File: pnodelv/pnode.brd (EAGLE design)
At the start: 50 x 23 mm, 42 parts, among them IC2 HTU21D, IC3 SI4012, J1 SWD_SHROUD_SMD

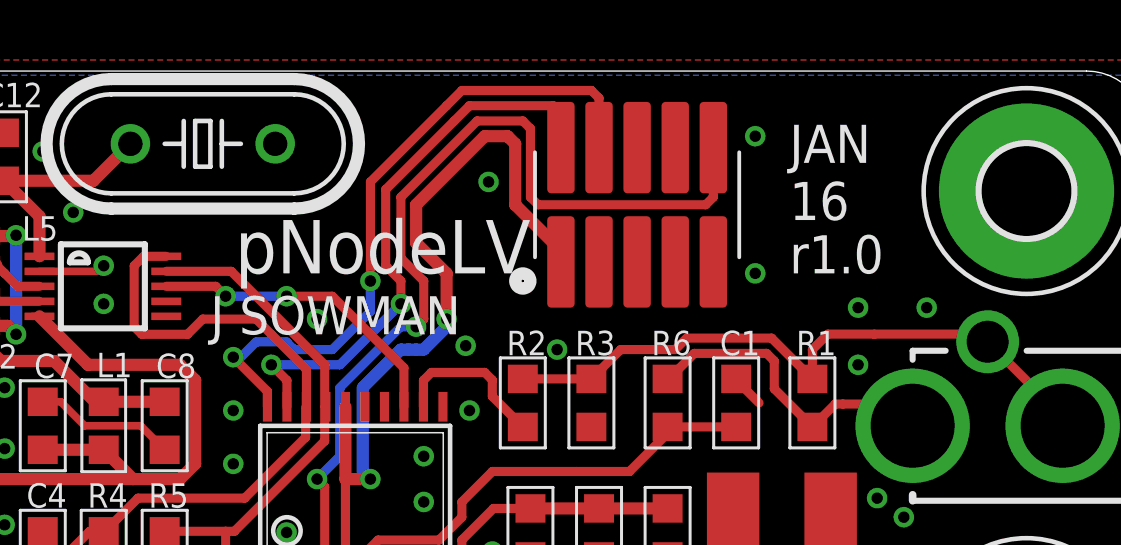
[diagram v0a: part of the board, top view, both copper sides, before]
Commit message: tidying silk again
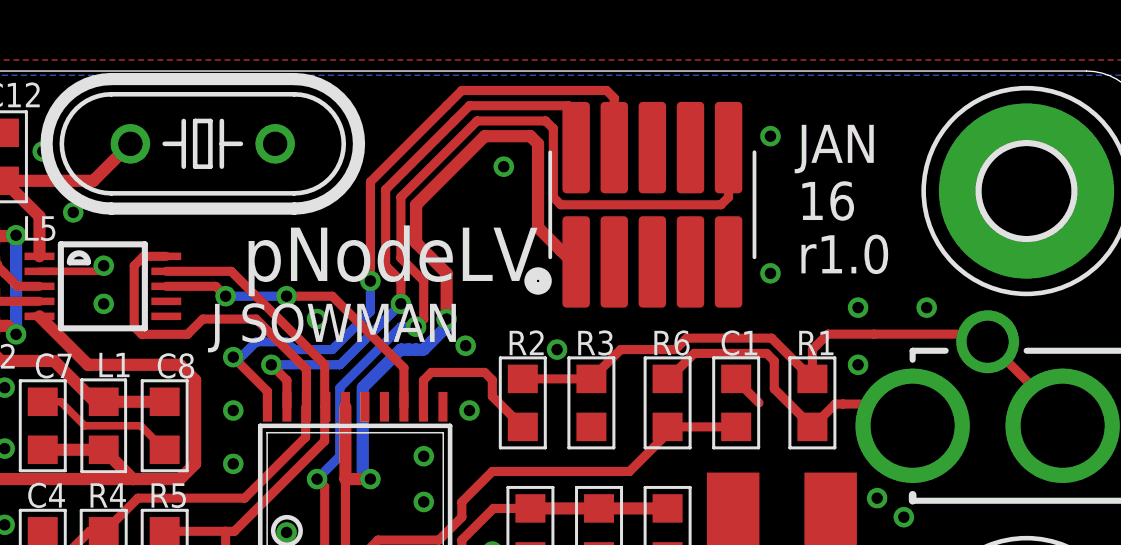
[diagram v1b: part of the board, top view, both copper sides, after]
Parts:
- moved J1 0.51 mm to (33.5, 18.5)
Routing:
- net +3V3: track 92.0 -> 92.6 mm
- net SWCLK: track 22.5 -> 23.0 mm
- net SWDAT: track 19.0 -> 19.6 mm
- net NRST: track 30.8 -> 31.3 mm
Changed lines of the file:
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@@
 <wire x1="50" y1="21" x2="48" y2="23" width="0" layer="20" curve="90"/>
 <text x="11.176" y="2.032" size="1.27" layer="21" font="vector" ratio="15" rot="R90">M0JSN</text>
-<text x="18.796" y="14.224" size="1.27" layer="21" font="vector" ratio="15">J SOWMAN</text>
-<text x="38.1" y="18.034" size="1.27" layer="21" font="vector" ratio="15">JAN
+<text x="18.796" y="13.97" size="1.27" layer="21" font="vector" ratio="15">J SOWMAN</text>
+<text x="38.354" y="18.034" size="1.27" layer="21" font="vector" ratio="15">JAN
 16</text>
 <text x="9.398" y="0.508" size="1.27" layer="21" font="vector" ratio="15" rot="R90">UKHASnet</text>
 <text x="36.83" y="0.254" size="1.27" layer="21" font="vector" ratio="15">1.5V</text>
-<text x="29.464" y="18.034" size="1.778" layer="21" font="vector" ratio="15" rot="R180">pNodeLV</text>
+<text x="29.718" y="17.78" size="1.778" layer="21" font="vector" ratio="15" rot="R180">pNodeLV</text>
 <text x="33.02" y="5.842" size="2.54" layer="22" font="vector" ratio="15" rot="MR0">pNodeLV</text>
 <text x="34.544" y="1.778" size="2.54" layer="22" font="vector" ratio="15" rot="MR0">J SOWMAN</text>
 <text x="9.652" y="18.542" size="1.27" layer="22" font="vector" ratio="15" rot="MR270">jonsowman.com</text>
-<text x="38.1" y="16.256" size="1.27" layer="21" font="vector" ratio="15">r1.0</text>
+<text x="38.354" y="16.256" size="1.27" layer="21" font="vector" ratio="15">r1.0</text>
 </plain>
 <attributes>
@@
 </element>
 <element name="L6" library="jonsowman" package="BOURNS_SDE0403A" value="4.7u" x="37.846" y="7.366"/>
-<element name="J1" library="dtb" package="SWD_SMD_SHROUD" value="SWD_SHROUD_SMD" x="33.02" y="18.542"/>
+<element name="J1" library="dtb" package="SWD_SMD_SHROUD" value="SWD_SHROUD_SMD" x="33.528" y="18.542"/>
 </elements>
 <signals>
@@
 <wire x1="36.322" y1="12.738" x2="36.322" y2="12.7" width="0.3048" layer="1"/>
 <wire x1="36.322" y1="12.7" x2="37.084" y2="11.938" width="0.3048" layer="1"/>
-<via x="28.067" y="19.304" extent="1-16" drill="0.381"/>
+<via x="28.575" y="19.812" extent="1-16" drill="0.381"/>
 <via x="27.305" y="13.843" extent="1-16" drill="0.381"/>
-<via x="36.957" y="20.828" extent="1-16" drill="0.381"/>
-<via x="36.957" y="16.256" extent="1-16" drill="0.381"/>
+<via x="37.465" y="20.828" extent="1-16" drill="0.381"/>
+<via x="37.465" y="16.256" extent="1-16" drill="0.381"/>
 </signal>
 <signal name="+3V3">
@@
 <wire x1="25.108" y1="1.956" x2="25.146" y2="1.994" width="0.4064" layer="1"/>
 <contactref element="J1" pad="1"/>
-<wire x1="30.48" y1="16.637" x2="30.48" y2="16.764" width="0.4064" layer="1"/>
-<wire x1="30.48" y1="16.637" x2="30.48" y2="17.018" width="0.4064" layer="1"/>
-<wire x1="30.48" y1="17.018" x2="28.956" y2="18.542" width="0.4064" layer="1"/>
-<wire x1="28.956" y1="18.542" x2="28.956" y2="20.574" width="0.4064" layer="1"/>
-<wire x1="28.956" y1="20.574" x2="28.702" y2="20.828" width="0.4064" layer="1"/>
-<wire x1="28.702" y1="20.828" x2="27.94" y2="20.828" width="0.4064" layer="1"/>
+<wire x1="30.48" y1="17.018" x2="29.718" y2="17.78" width="0.4064" layer="1"/>
+<wire x1="29.718" y1="17.78" x2="29.718" y2="20.574" width="0.4064" layer="1"/>
+<wire x1="29.718" y1="20.574" x2="29.464" y2="20.828" width="0.4064" layer="1"/>
+<wire x1="29.464" y1="20.828" x2="27.94" y2="20.828" width="0.4064" layer="1"/>
 <wire x1="27.94" y1="20.828" x2="25.654" y2="18.542" width="0.4064" layer="1"/>
 <wire x1="25.654" y1="18.542" x2="25.654" y2="17.272" width="0.4064" layer="1"/>
@@
 <via x="26.67" y="14.732" extent="1-16" drill="0.381"/>
 <wire x1="26.67" y1="14.732" x2="26.67" y2="14.478" width="0.4064" layer="16"/>
+<wire x1="30.988" y1="16.637" x2="30.861" y2="16.637" width="0.4064" layer="1"/>
+<wire x1="30.861" y1="16.637" x2="30.48" y2="17.018" width="0.4064" layer="1"/>
 </signal>
 <signal name="SCL">
@@
 <contactref element="J1" pad="2"/>
 <wire x1="26.924" y1="21.336" x2="27.432" y2="21.844" width="0.3048" layer="1"/>
-<wire x1="27.432" y1="21.844" x2="30.226" y2="21.844" width="0.3048" layer="1"/>
-<wire x1="30.226" y1="21.844" x2="30.48" y2="21.59" width="0.3048" layer="1"/>
-<wire x1="30.48" y1="21.59" x2="30.48" y2="20.447" width="0.3048" layer="1"/>
+<wire x1="27.432" y1="21.844" x2="30.734" y2="21.844" width="0.3048" layer="1"/>
+<wire x1="30.734" y1="21.844" x2="30.988" y2="21.59" width="0.3048" layer="1"/>
+<wire x1="30.988" y1="21.59" x2="30.988" y2="20.447" width="0.3048" layer="1"/>
 </signal>
 <signal name="SWCLK">
@@
 <contactref element="J1" pad="4"/>
 <wire x1="26.67" y1="21.844" x2="27.178" y2="22.352" width="0.3048" layer="1"/>
-<wire x1="27.178" y1="22.352" x2="31.496" y2="22.352" width="0.3048" layer="1"/>
-<wire x1="31.496" y1="22.352" x2="31.75" y2="22.098" width="0.3048" layer="1"/>
-<wire x1="31.75" y1="22.098" x2="31.75" y2="20.447" width="0.3048" layer="1"/>
+<wire x1="27.178" y1="22.352" x2="32.004" y2="22.352" width="0.3048" layer="1"/>
+<wire x1="32.004" y1="22.352" x2="32.258" y2="22.098" width="0.3048" layer="1"/>
+<wire x1="32.258" y1="22.098" x2="32.258" y2="20.447" width="0.3048" layer="1"/>
 </signal>
 <signal name="NRST">
@@
 <wire x1="25.146" y1="16.764" x2="25.146" y2="18.796" width="0.3048" layer="1"/>
 <wire x1="25.146" y1="18.796" x2="27.686" y2="21.336" width="0.3048" layer="1"/>
-<wire x1="27.686" y1="21.336" x2="29.21" y2="21.336" width="0.3048" layer="1"/>
-<wire x1="29.21" y1="21.336" x2="29.464" y2="21.082" width="0.3048" layer="1"/>
-<wire x1="29.464" y1="21.082" x2="29.464" y2="18.796" width="0.3048" layer="1"/>
-<wire x1="29.464" y1="18.796" x2="29.718" y2="18.542" width="0.3048" layer="1"/>
-<wire x1="29.718" y1="18.542" x2="35.306" y2="18.542" width="0.3048" layer="1"/>
-<wire x1="35.306" y1="18.542" x2="35.56" y2="18.796" width="0.3048" layer="1"/>
-<wire x1="35.56" y1="18.796" x2="35.56" y2="20.447" width="0.3048" layer="1"/>
+<wire x1="27.686" y1="21.336" x2="29.972" y2="21.336" width="0.3048" layer="1"/>
+<wire x1="29.972" y1="21.336" x2="30.226" y2="21.082" width="0.3048" layer="1"/>
+<wire x1="30.226" y1="21.082" x2="30.226" y2="18.796" width="0.3048" layer="1"/>
+<wire x1="30.226" y1="18.796" x2="30.48" y2="18.542" width="0.3048" layer="1"/>
+<wire x1="30.48" y1="18.542" x2="35.814" y2="18.542" width="0.3048" layer="1"/>
+<wire x1="35.814" y1="18.542" x2="36.068" y2="18.796" width="0.3048" layer="1"/>
+<wire x1="36.068" y1="18.796" x2="36.068" y2="20.447" width="0.3048" layer="1"/>
 <wire x1="25.908" y1="16.002" x2="25.908" y2="14.732" width="0.3048" layer="1"/>
 <wire x1="25.908" y1="14.732" x2="25.654" y2="14.478" width="0.3048" layer="1"/>
